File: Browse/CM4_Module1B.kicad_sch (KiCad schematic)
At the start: 10 parts, among them J3 179-UJ20CHC4SMTTR

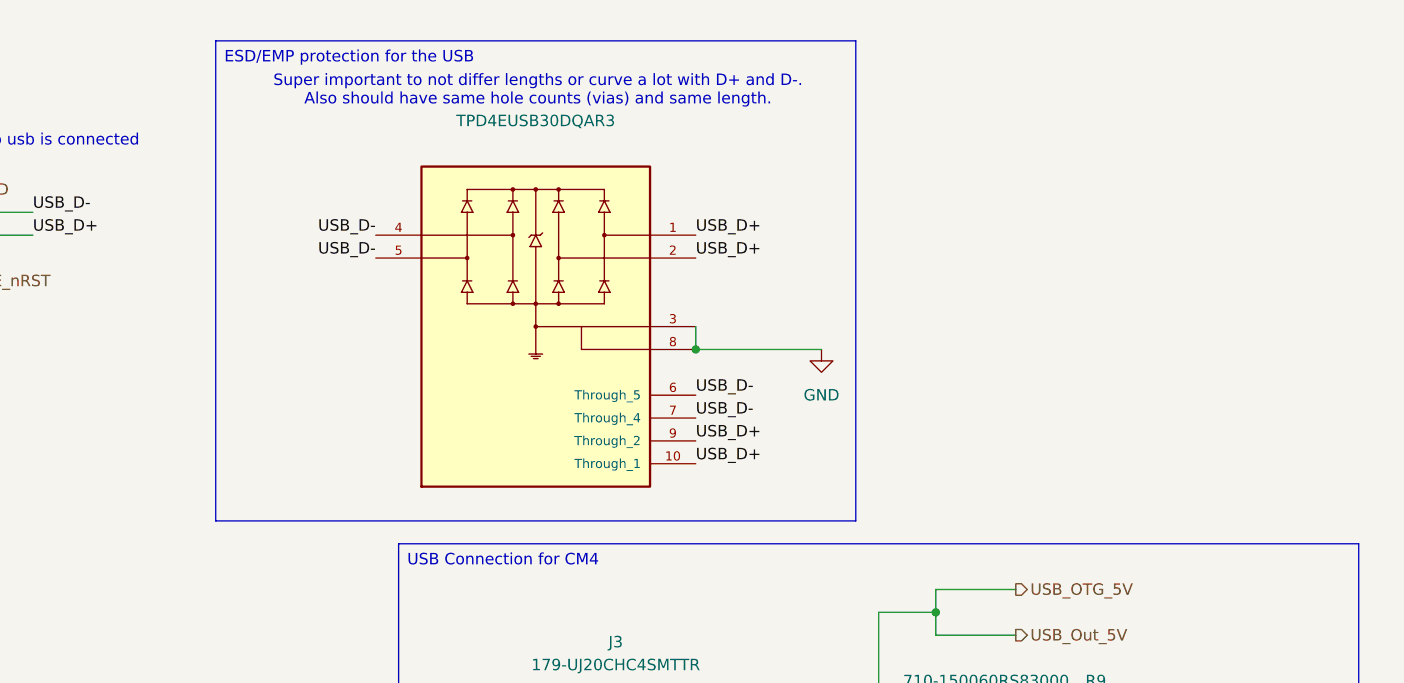
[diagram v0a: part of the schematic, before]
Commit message: Deploying to gh-pages from @ Nautilus-UUV/nautilus-mainboard-PCB@62d9beca31554f779583bfc3c938b3f82a581309 🚀
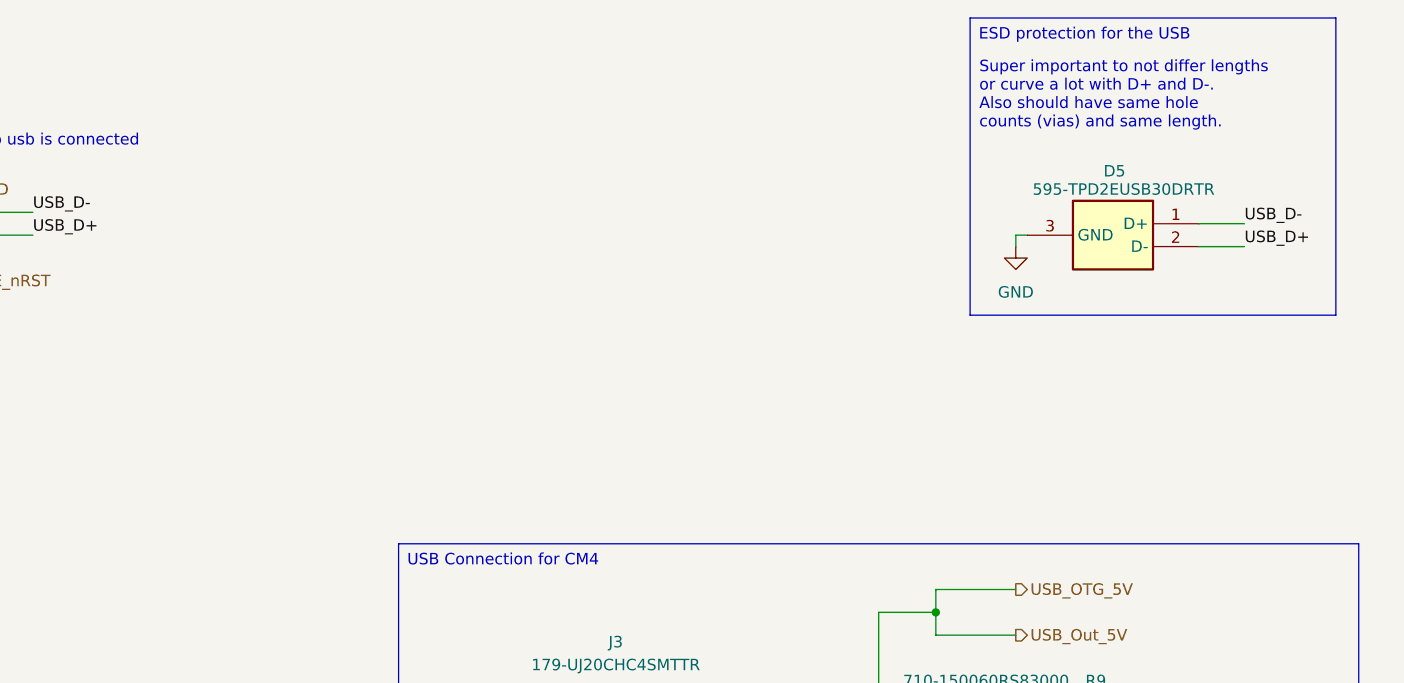
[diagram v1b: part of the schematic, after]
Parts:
- removed TPD4EUSB30DQAR3: ~, dz_con:IC_TPD4EUSB30DQAR, symbol #dzdb:s_misc/IC-ESD-TPD4EUSB30
- added D5: 595-TPD2EUSB30DRTR, dz_dio:TI_Prot_TPD2EUSB30DRTR, symbol #dzdb:s_dio/TEXA-595-TPD2EUSB30DRTR
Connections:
- net GND: now also D5.3 (GND)
- net USB_D+: now also D5.2 (D-)
- net USB_D-: now also D5.1 (D+)

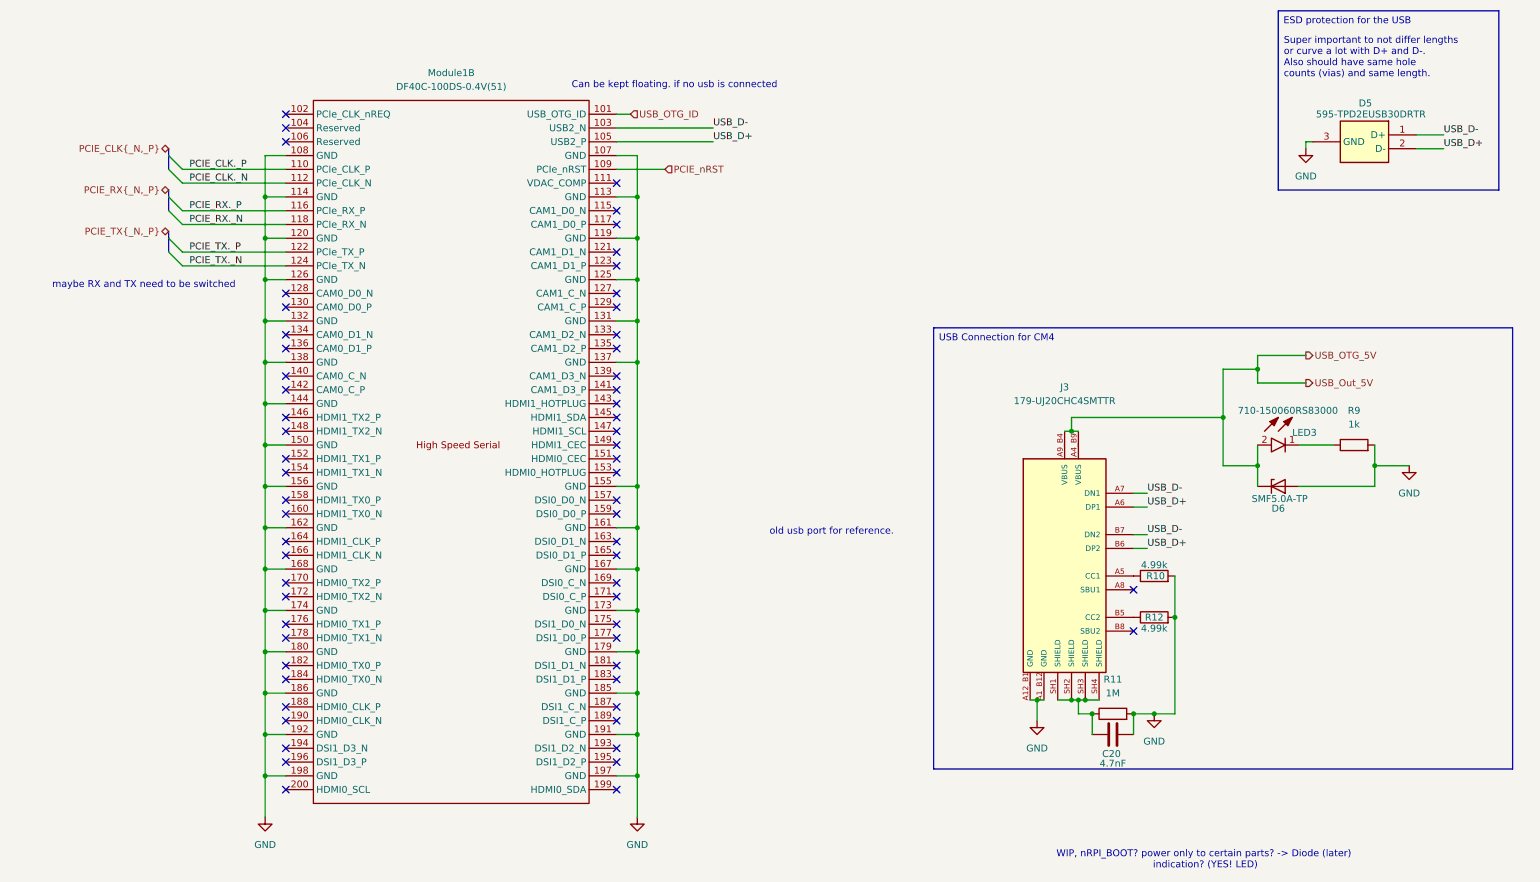
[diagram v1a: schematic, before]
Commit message: Deploying to gh-pages from @ Nautilus-UUV/nautilus-mainboard-PCB@5f5fdd9436d408a604bb268d740c0ac7ce1f5af5 🚀
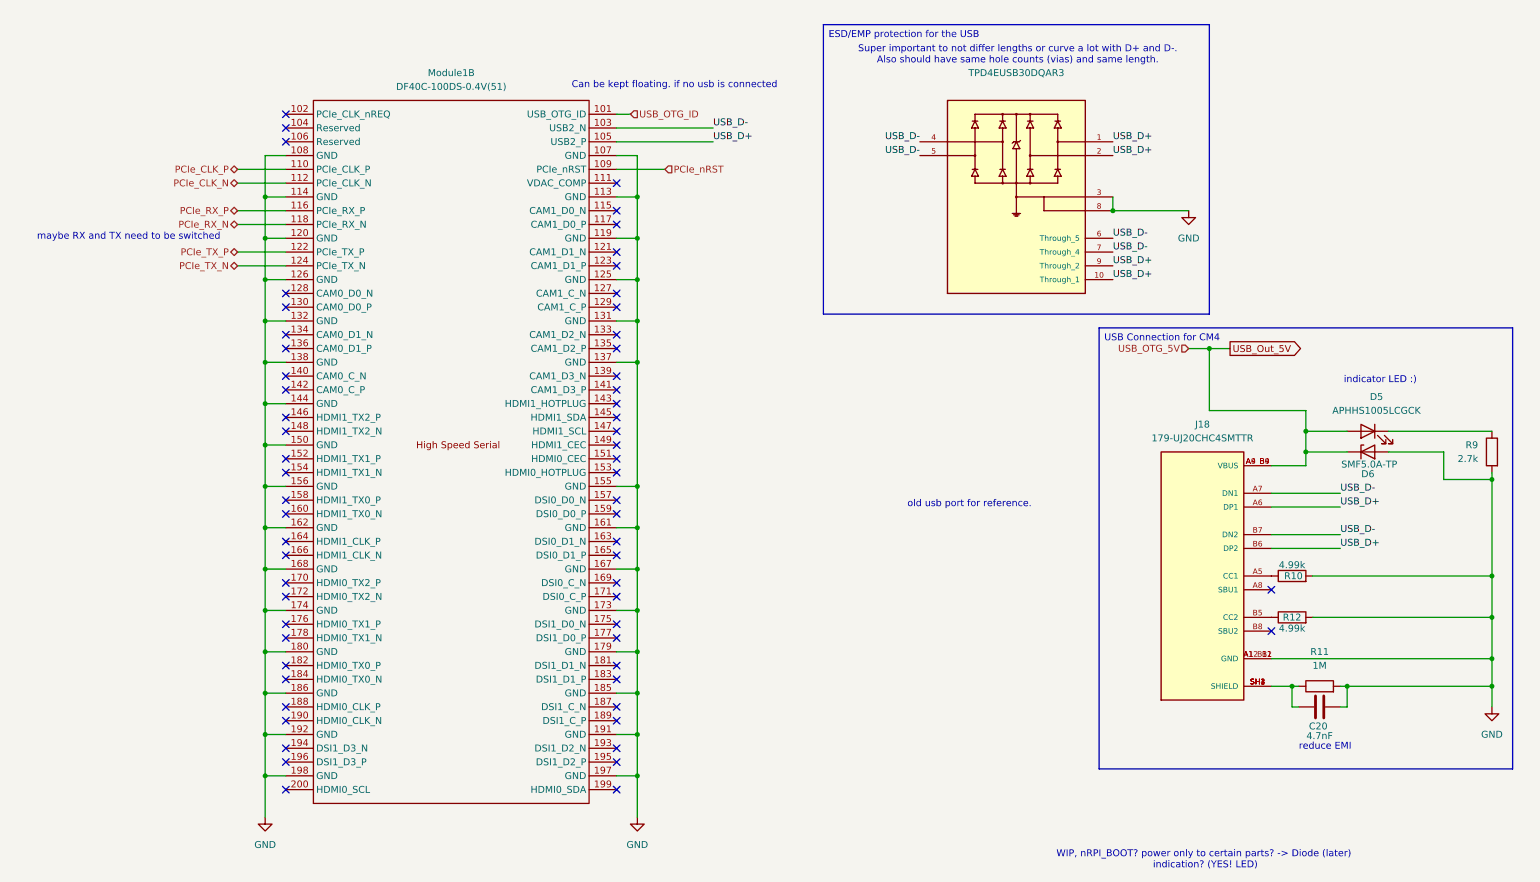
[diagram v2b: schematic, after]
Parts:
- removed D5: 595-TPD2EUSB30DRTR, dz_dio:TI_Prot_TPD2EUSB30DRTR, symbol #dzdb:s_dio/TEXA-595-TPD2EUSB30DRTR
- removed J3: 179-UJ20CHC4SMTTR, dz_con:CON_Samesky_CUI_UJ20-C-H-C-4-SMT-TR, symbol #dzdb:s_con/SAME-179-UJ20CHC4SMTTR
- removed LED3: 710-150060RS83000, dz_dio:Wuerth_LED_150060RS83000, symbol #dzdb:s_dio/D-WURT-710-150060RS83000
- removed R9: 1k, Resistor_SMD:R_0603_1608Metric, symbol #dzdb:g_res/R-1k-0603
- added D5: APHHS1005LCGCK, LED_SMD:LED_0402_1005Metric, symbol #dzdb:s_dio/D-KIN-APHHS1005LCGCK
- added J18: 179-UJ20CHC4SMTTR, dz_con:CON_Samesky_CUI_UJ20-C-H-C-4-SMT-TR, symbol #dzdb:s_con/SAME-179-UJ20CHC4SMTTR
- added R9: 2.7k, Resistor_SMD:R_0603_1608Metric, symbol #dzdb:g_res/R-2.7k-0603
- added TPD4EUSB30DQAR3: ~, dz_con:IC_TPD4EUSB30DQAR, symbol #dzdb:s_misc/IC-ESD-TPD4EUSB30
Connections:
- net GND: now also J18.A12_B1 (GND), J18.A1_B12 (GND), R9.2, TPD4EUSB30DQAR3.3, TPD4EUSB30DQAR3.8
- net USB_D+: now also J18.A6 (DP1), J18.B6 (DP2), TPD4EUSB30DQAR3.1, TPD4EUSB30DQAR3.10 (Through_1), TPD4EUSB30DQAR3.2, TPD4EUSB30DQAR3.9 (Through_2)
- net USB_D-: now also J18.A7 (DN1), J18.B7 (DN2), TPD4EUSB30DQAR3.4, TPD4EUSB30DQAR3.5, TPD4EUSB30DQAR3.6 (Through_5), TPD4EUSB30DQAR3.7 (Through_4)
- net at C20.2, R11.1: now also J18.SH1 (SHIELD), J18.SH2 (SHIELD), J18.SH3 (SHIELD), J18.SH4 (SHIELD)
- net at R10.1: now also J18.A5 (CC1)
- net at R12.1: now also J18.B5 (CC2)
- net PCIE_CLK._N renamed PCIe_CLK_N
- net PCIE_CLK._P renamed PCIe_CLK_P
- net PCIE_RX._N renamed PCIe_RX_N
- net PCIE_RX._P renamed PCIe_RX_P
- net PCIE_TX._N renamed PCIe_TX_N
- net PCIE_TX._P renamed PCIe_TX_P
- net PCIE_nRST renamed PCIe_nRST
- net USB_OTG_5V renamed USB_Out_5V
- net USB_Out_5V: now also D5.2 (A), J18.A4_B9 (VBUS), J18.A9_B4 (VBUS)
- new net: D5.1 (K), R9.1
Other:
- note added: "indicator LED :)"
- note added: "reduce EMI"
- company: Davide -> (none)
- title: Nautilus_Mainboard -> (none)
- moved on the sheet: C20, D6, R10, R11, R12

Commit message: Deploying to gh-pages from @ Nautilus-UUV/nautilus-mainboard-PCB@f1dd6ce1e57c066b805694b10777c719502cca87 🚀
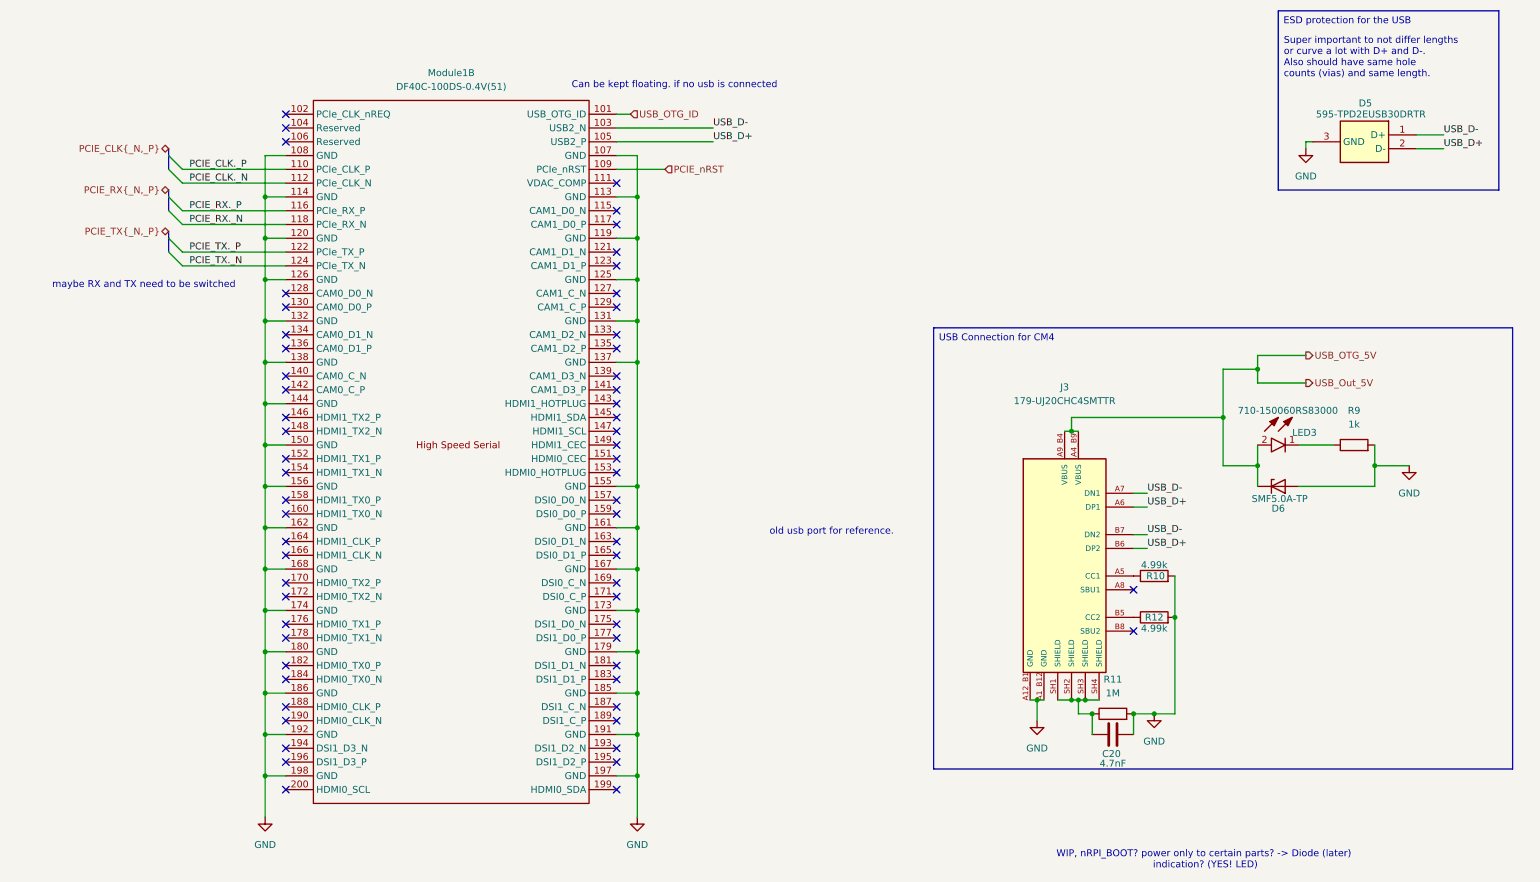
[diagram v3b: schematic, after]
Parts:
- removed D5: APHHS1005LCGCK, LED_SMD:LED_0402_1005Metric, symbol #dzdb:s_dio/D-KIN-APHHS1005LCGCK
- removed J18: 179-UJ20CHC4SMTTR, dz_con:CON_Samesky_CUI_UJ20-C-H-C-4-SMT-TR, symbol #dzdb:s_con/SAME-179-UJ20CHC4SMTTR
- removed R9: 2.7k, Resistor_SMD:R_0603_1608Metric, symbol #dzdb:g_res/R-2.7k-0603
- removed TPD4EUSB30DQAR3: ~, dz_con:IC_TPD4EUSB30DQAR, symbol #dzdb:s_misc/IC-ESD-TPD4EUSB30
- added D5: 595-TPD2EUSB30DRTR, dz_dio:TI_Prot_TPD2EUSB30DRTR, symbol #dzdb:s_dio/TEXA-595-TPD2EUSB30DRTR
- added J3: 179-UJ20CHC4SMTTR, dz_con:CON_Samesky_CUI_UJ20-C-H-C-4-SMT-TR, symbol #dzdb:s_con/SAME-179-UJ20CHC4SMTTR
- added LED3: 710-150060RS83000, dz_dio:Wuerth_LED_150060RS83000, symbol #dzdb:s_dio/D-WURT-710-150060RS83000
- added R9: 1k, Resistor_SMD:R_0603_1608Metric, symbol #dzdb:g_res/R-1k-0603
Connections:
- net GND: now also D5.3 (GND), J3.A12_B1 (GND), J3.A1_B12 (GND), R9.2
- net USB_D+: now also D5.2 (D-), J3.A6 (DP1), J3.B6 (DP2)
- net USB_D-: now also D5.1 (D+), J3.A7 (DN1), J3.B7 (DN2)
- net at C20.2, R11.1: now also J3.SH1 (SHIELD), J3.SH2 (SHIELD), J3.SH3 (SHIELD), J3.SH4 (SHIELD)
- net at R10.1: now also J3.A5 (CC1)
- net at R12.1: now also J3.B5 (CC2)
- net PCIe_CLK_N renamed PCIE_CLK._N
- net PCIe_CLK_P renamed PCIE_CLK._P
- net PCIe_RX_N renamed PCIE_RX._N
- net PCIe_RX_P renamed PCIE_RX._P
- net PCIe_TX_N renamed PCIE_TX._N
- net PCIe_TX_P renamed PCIE_TX._P
- net PCIe_nRST renamed PCIE_nRST
- net USB_Out_5V renamed USB_OTG_5V
- net USB_OTG_5V: now also J3.A4_B9 (VBUS), J3.A9_B4 (VBUS), LED3.2 (A)
- new net: LED3.1 (K), R9.1
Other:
- note removed: "indicator LED :)"
- note removed: "reduce EMI"
- company: (none) -> Davide
- title: (none) -> Nautilus_Mainboard
- moved on the sheet: C20, D6, R10, R11, R12
